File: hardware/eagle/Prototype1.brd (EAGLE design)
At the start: 100 x 80 mm, 26 parts, among them U1 ARDUINO_SHIELDLABEL

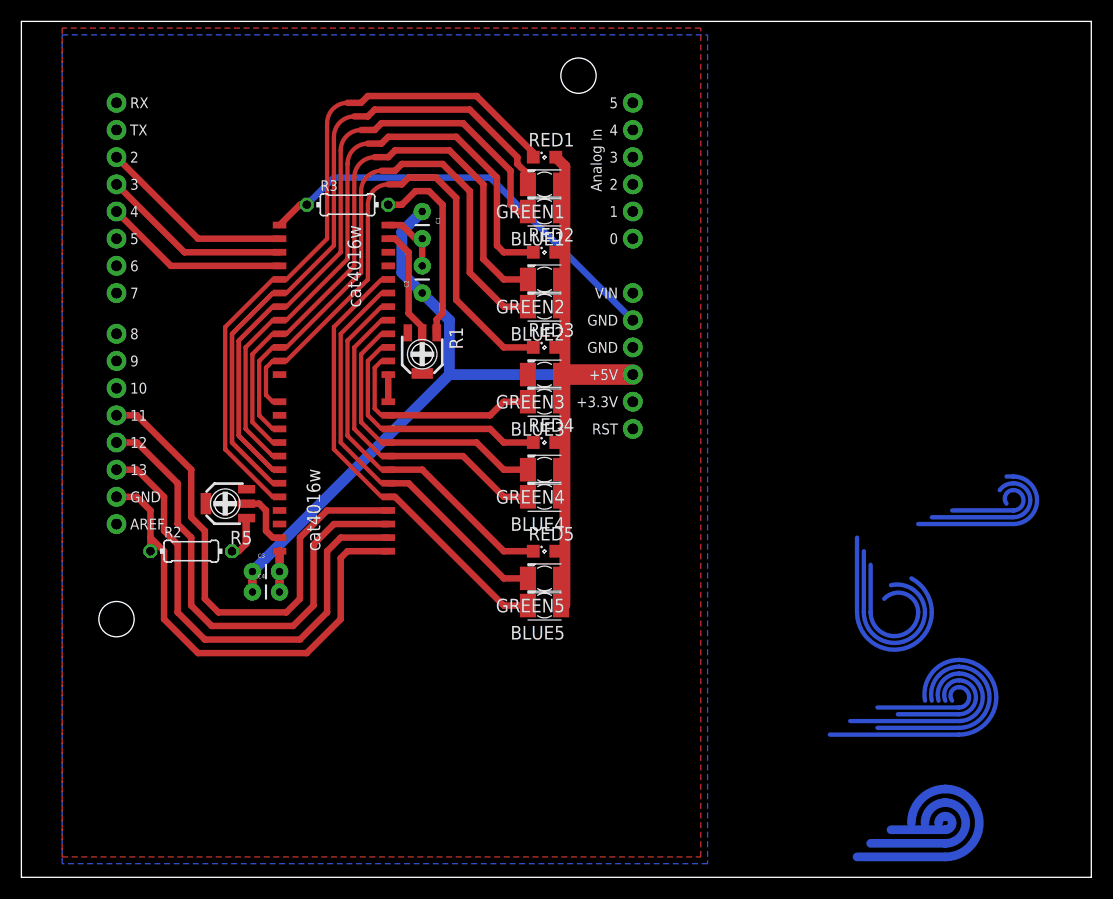
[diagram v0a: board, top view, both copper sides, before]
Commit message: finished Prototype1, created gerber
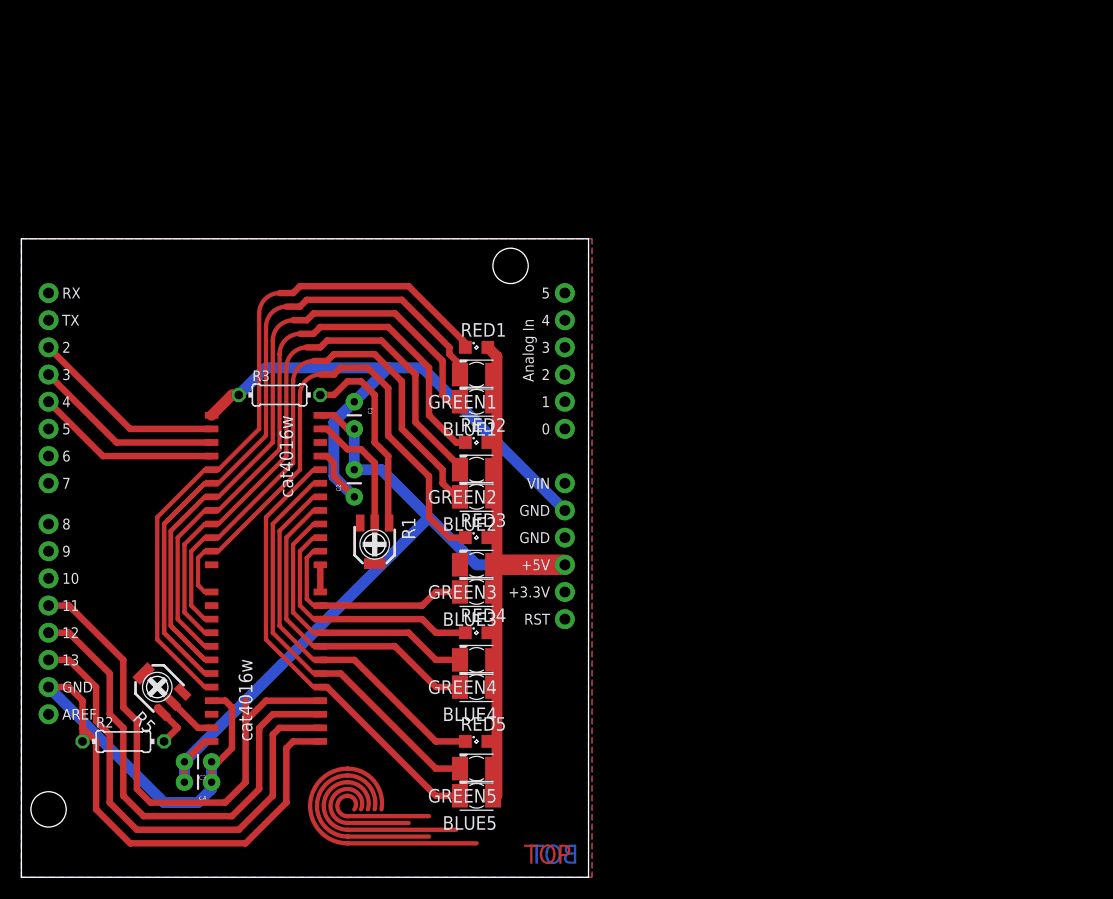
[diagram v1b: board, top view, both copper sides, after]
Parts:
- moved C2 20.1 mm to (31.1, 35.6)
- moved U$3 18.9 mm to (22.9, 19.7)
- moved BLUE2 18.9 mm to (42.5, 35.6)
- moved BLUE3 18.9 mm to (42.5, 26.7)
- moved BLUE4 18.9 mm to (42.5, 17.8)
- moved GREEN2 18.9 mm to (42.5, 38.1)
- moved GREEN3 18.9 mm to (42.5, 29.2)
- moved GREEN4 18.9 mm to (42.5, 20.3)
- moved GREEN5 18.9 mm to (42.5, 10.2)
- moved R2 18.9 mm to (9.53, 12.7)
- moved R3 18.9 mm to (24.1, 45.1)
- moved RED1 18.9 mm to (42.5, 49.5)
- moved RED2 18.9 mm to (42.5, 40.6)
- moved RED3 18.9 mm to (42.5, 31.8)
- moved RED4 18.9 mm to (42.5, 22.9)
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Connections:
- removed net N$1: C1.2, C2.2, U$2.24
- removed net N$6: C3.2, C4.2, U$3.24
- net +5V: now also C1.2, C2.2, C3.2, C4.2, U$2.24, U$3.24; no longer C1.1, C2.1, C3.1, C4.1
- net GND: now also C1.1, C2.1, C3.1, C4.1, U$2.21, U$3.21
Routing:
- net GND: track 85.6 -> 153.4 mm
- net N$45: track 19.1 -> 0.00 mm
- net N$34: track 17.7 -> 0.00 mm
- net N$33: track 15.5 -> 0.00 mm
- net N$48: track 14.0 -> 0.00 mm
- net N$44: track 13.5 -> 0.00 mm
- net N$32: track 12.3 -> 0.00 mm
- net N$47: track 12.2 -> 0.00 mm
- net N$46: track 9.04 -> 0.00 mm
- net +5V: track 112.2 -> 119.6 mm
- net N$43: track 7.25 -> 0.00 mm
- net N$1: track 6.24 -> 0.00 mm
- net N$6: track 3.81 -> 0.00 mm
- net N$4: track 9.94 -> 12.1 mm
- net N$3: track 6.57 -> 4.49 mm
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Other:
- board size 100 x 80 mm -> 53 x 59.7 mm
- board text added: "BOT"
- board text added: "TOP"
